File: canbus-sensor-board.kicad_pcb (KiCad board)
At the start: 4 copper layers, 32 x 49 mm, 48 parts, among them J1 CAN IO, J2 CAN Term, J3 POWER IN, J4 Debug, J5 I2C2 IO, J6 I2C1 IO, Q1 2N7002, Q2 2N7002, Q3 2N7002, Q4 2N7002, SW1 Reset, SW2 Boot, U1 MCP2551-I-SN, U3 AMS1117-3.3, U4 STM32F103C8Tx

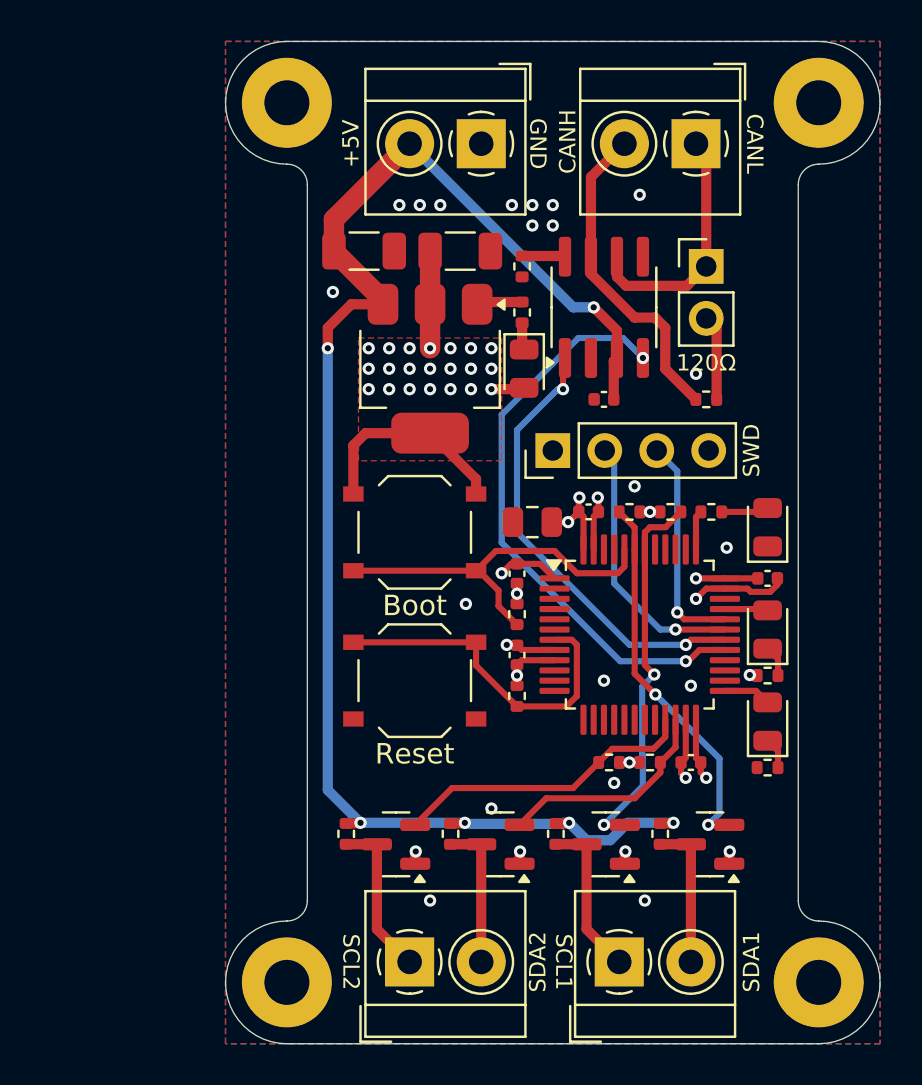
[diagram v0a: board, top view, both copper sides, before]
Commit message: Update board to rev 3 (we do not talk about rev 2)
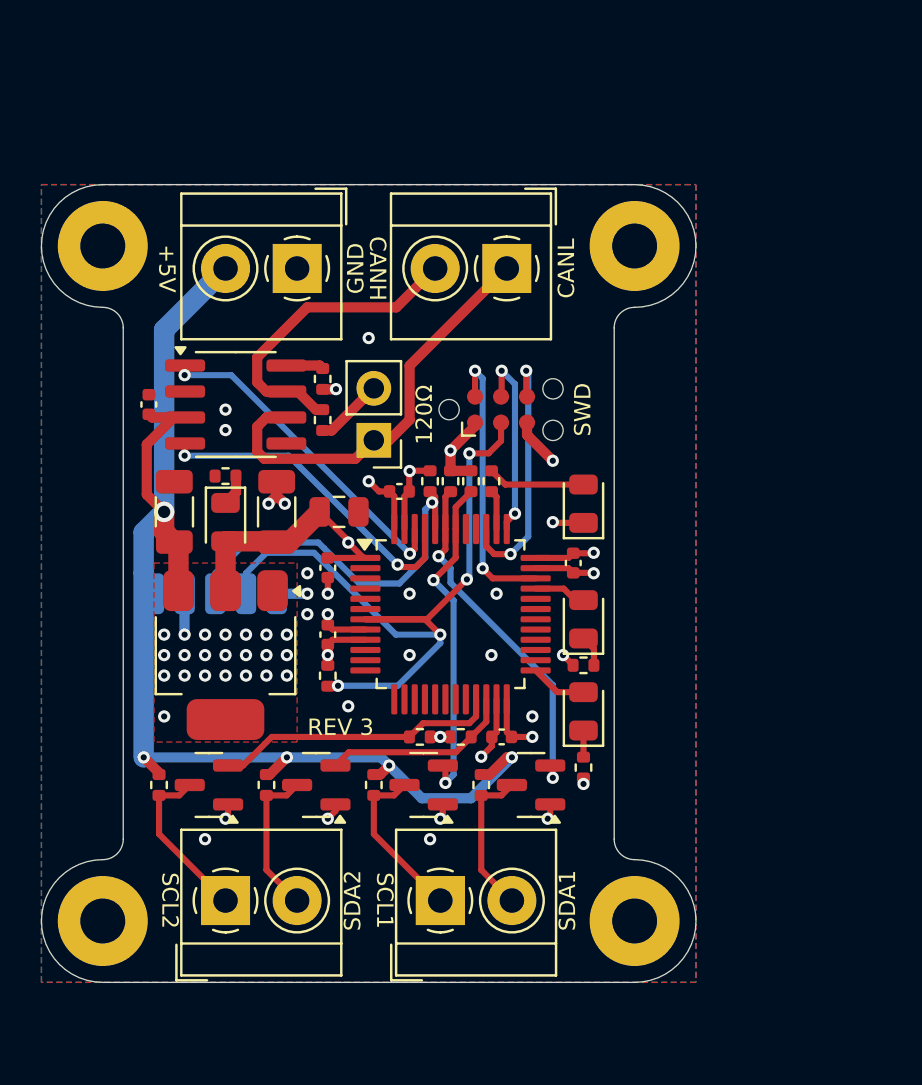
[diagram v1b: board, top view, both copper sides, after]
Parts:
- removed SW1: Reset, Button_Switch_SMD:SW_Push_1P1T_XKB_TS-1187A
- removed SW2: Boot, Button_Switch_SMD:SW_Push_1P1T_XKB_TS-1187A
- added J10: Conn_01x01, Connector_Wire:SolderWirePad_1x01_SMD_1x2mm, B.Cu at (31.5, 50.0)
- added J11: Conn_01x01, Connector_Wire:SolderWirePad_1x01_SMD_1x2mm, B.Cu at (27.0, 50.0)
- added J7: Conn_01x01, Connector_Wire:SolderWirePad_1x01_SMD_1x2mm, B.Cu at (28.5, 50.0)
- added J8: Conn_ARM_SWD_TagConnect_TC2030-NL, Connector:Tag-Connect_TC2030-IDC-NL_2x03_P1.27mm_Vertical, F.Cu at (42.5, 41.0)
- added J9: Conn_01x01, Connector_Wire:SolderWirePad_1x01_SMD_1x2mm, B.Cu at (30.0, 50.0)
- J4: value Debug -> Conn_01x01; footprint Connector_PinHeader_2.54mm:PinHeader_1x04_P2.54mm_Vertical -> Connector_Wire:SolderWirePad_1x01_SMD_1x2mm; moved to B.Cu
- moved C5 22.3 mm to (25.2, 40.8), turned to 90 degrees
- moved J4 20.7 mm to (25.5, 50.0), turned to 180 degrees
- moved R1 18.8 mm to (33.8, 41.5), turned to -90 degrees
- moved U1 18.6 mm to (29.5, 40.8), turned to 0 degrees
- moved J2 18.3 mm to (36.2, 42.5), turned to 180 degrees
- moved U3 17.2 mm to (29.0, 53.0)
- moved R5 16.6 mm to (29.0, 44.2), turned to 0 degrees
- moved D1 16.4 mm to (29.0, 46.5)
- moved C6 15.8 mm to (26.5, 46.0), turned to 90 degrees
- moved C7 15.6 mm to (31.5, 46.0), turned to 90 degrees
- moved H1 11.4 mm to (23.0, 33.0)
- moved H2 11.4 mm to (49.0, 33.0)
- moved R2 11.2 mm to (33.8, 39.5)
- moved J1 11.1 mm to (42.8, 34.1)
- moved J3 10.9 mm to (32.5, 34.1)
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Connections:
- J4 pad 1: GND -> +5V
- R3 pad 1: +3.3V -> NRST
- R3 pad 2: NRST -> +3.3V
- U4 pad 29: CAN_RX -> unconnected-(U4-PA8-Pad29)
- U4 pad 30: CAN_TX -> unconnected-(U4-PA9-Pad30)
- U4 pad 31: SYS_SWDIO -> unconnected-(U4-PA10-Pad31)
- U4 pad 32: SYS_SWCLK -> unconnected-(U4-PA11-Pad32)
- U4 pad 34: unconnected-(U4-PA13-Pad34) -> SWDIO
- U4 pad 37: DEBUG_LED1 -> SWCLK
- U4 pad 38: unconnected-(U4-PA15-Pad38) -> DEBUG_LED1
- U4 pad 39: unconnected-(U4-PB3-Pad39) -> SWO
- U4 pad 45: unconnected-(U4-PB8-Pad45) -> CAN_RX
- U4 pad 46: unconnected-(U4-PB9-Pad46) -> CAN_TX
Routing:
- net NRST: track 16.8 -> 38.0 mm, vias 0 -> 4
- net SWDIO: track 0.00 -> 13.9 mm, vias 0 -> 2
- net SYS_SWDIO: track 13.0 -> 0.00 mm, vias 1 -> 0
- net SWO: track 0.00 -> 12.8 mm, vias 0 -> 2
- net CAN_RX: track 28.7 -> 16.2 mm
- net +5V: track 74.6 -> 62.5 mm, vias 6 -> 5
- net SYS_SWCLK: track 10.8 -> 0.00 mm, vias 1 -> 0
- net SWCLK: track 0.00 -> 9.45 mm, vias 0 -> 2
- net CANL: track 12.1 -> 20.6 mm
- net CAN_TX: track 22.2 -> 16.4 mm
- net GND: track 16.4 -> 22.1 mm, vias 26 -> 27
- net +3.3V: track 37.3 -> 34.7 mm, vias 33 -> 32
- net Net-(D2-A): track 2.32 -> 4.78 mm
- net I2C1_SCL: track 18.8 -> 16.5 mm
- net I2C2_SDA: track 10.8 -> 9.36 mm
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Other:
- board size 32 x 49 mm -> 32 x 39 mm
- board text added: "3.3V"
- board text added: "5V"
- board text added: "BOOT"
- board text added: "CANBUS SENSOR BOARD REV 3 © 2024 David Flemström"
- board text added: "REV 3"
- board text added: "~{RST}"
- board text removed: "Boot"
- board text removed: "Reset"
